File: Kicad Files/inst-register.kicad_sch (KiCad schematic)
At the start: 20 parts, among them U32 74LS245, U33 74LS173, U34 74LS173

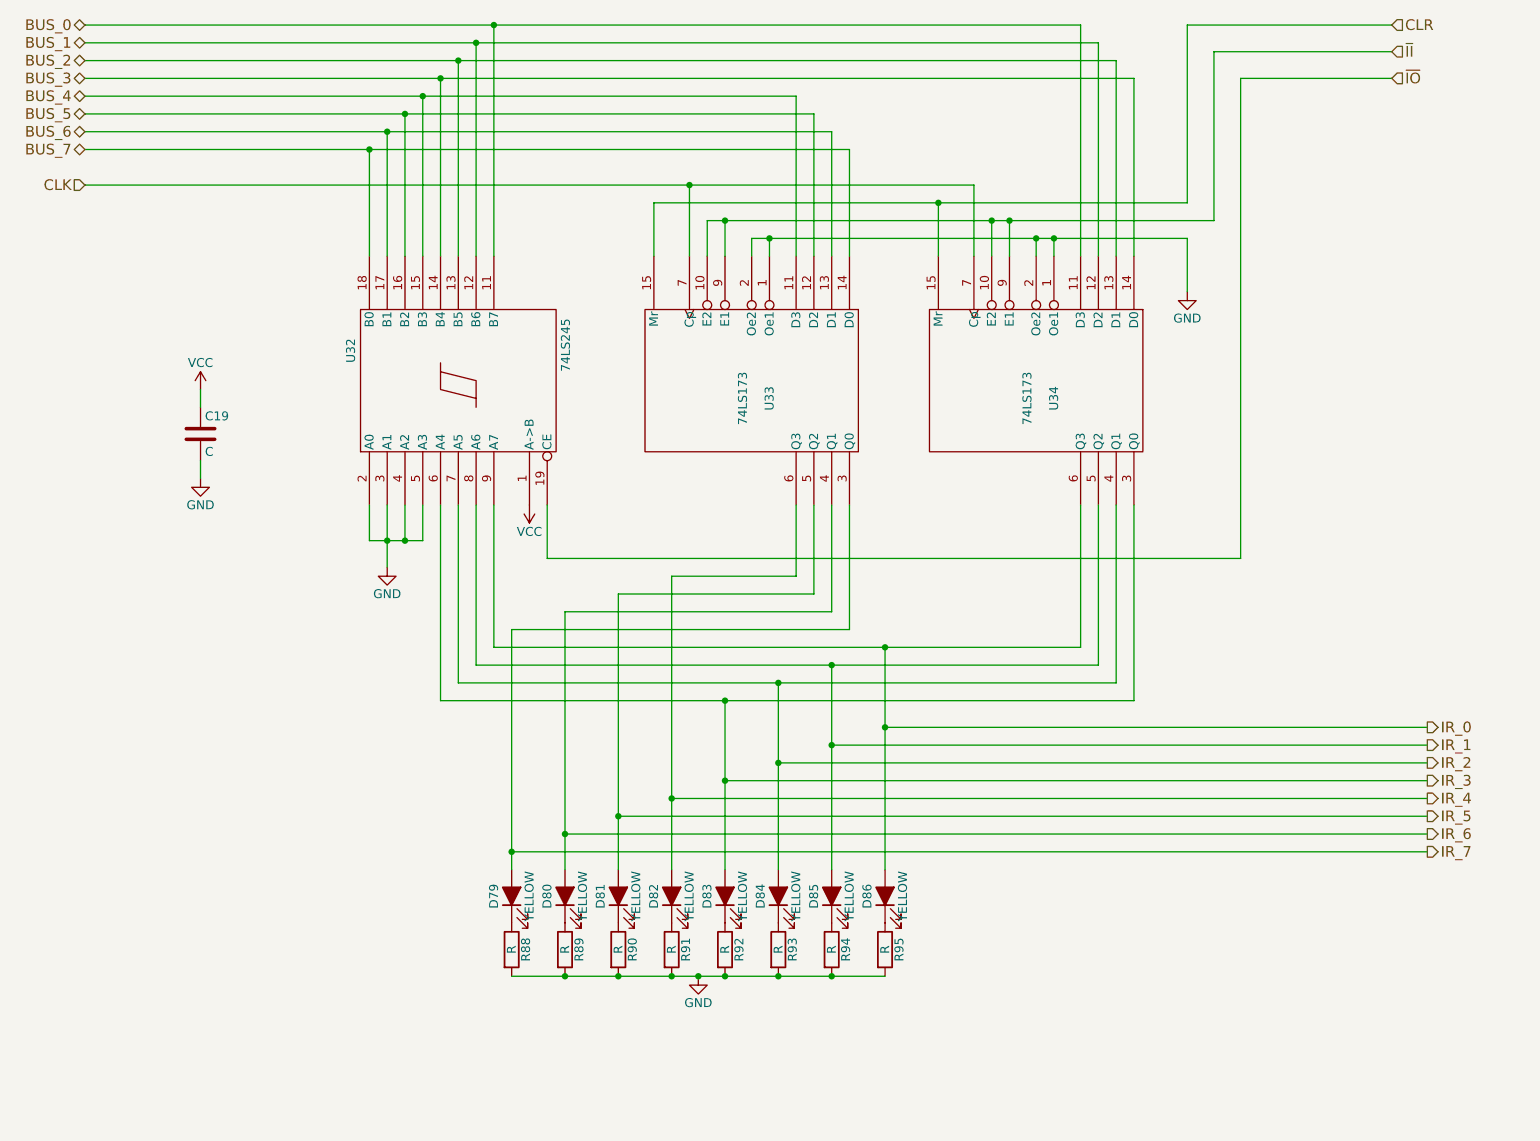
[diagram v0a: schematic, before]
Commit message: updated library
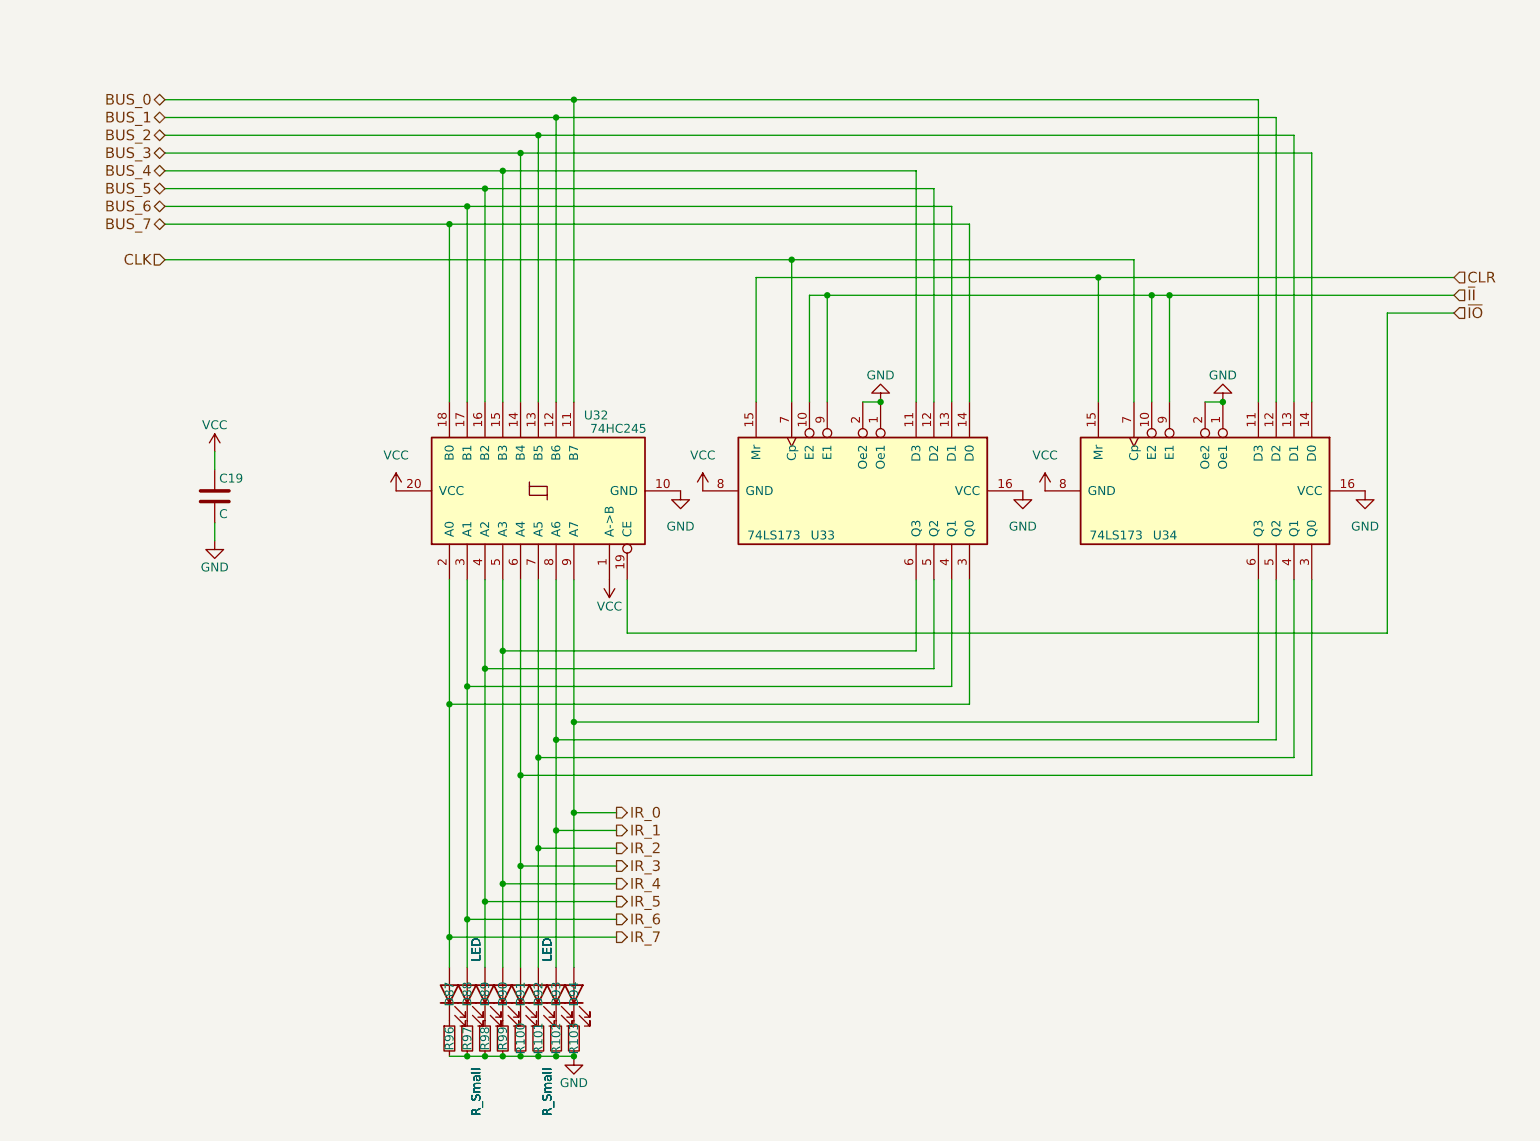
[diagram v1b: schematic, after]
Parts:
- removed D79, D80, D81, D82, D83, D84, D85, D86: YELLOW, LED_THT:LED_D5.0mm, symbol 8bit-computer-rescue:LED_ALT-Device
- removed R88, R89, R90, R91, R92, R93, R94, R95: R, Resistor_THT:R_Axial_DIN0207_L6.3mm_D2.5mm_P7.62mm_Horizontal, symbol Device:R
- removed U32: 74LS245, Package_DIP:DIP-20_W7.62mm, symbol 8bit-computer-rescue:74LS245-8bit-computer-rescue
- removed U33, U34: 74LS173, Package_DIP:DIP-16_W7.62mm, symbol 8bit-computer-rescue:74LS173-8bit-computer-rescue
- added D87, D88, D89, D90, D91, D92, D93, D94: LED, symbol Device:LED
- added R100, R101, R102, R103, R96, R97, R98, R99: R_Small, symbol Device:R_Small
- added U32: 74HC245, symbol 74xx:74HC245
- added U33, U34: 74LS173, symbol 74xx:74LS173
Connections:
- net BUS_0: now also U32.11 (B7), U34.11 (D3)
- net BUS_1: now also U32.12 (B6), U34.12 (D2)
- net BUS_2: now also U32.13 (B5), U34.13 (D1)
- net BUS_3: now also U32.14 (B4), U34.14 (D0)
- net BUS_4: now also U32.15 (B3), U33.11 (D3)
- net BUS_5: now also U32.16 (B2), U33.12 (D2)
- net BUS_6: now also U32.17 (B1), U33.13 (D1)
- net BUS_7: now also U32.18 (B0), U33.14 (D0)
- net CLK: now also U33.7 (Cp), U34.7 (Cp)
- net CLR: now also U33.15 (Mr), U34.15 (Mr)
- net GND: now also R100.2, R101.2, R102.2, R103.2, R96.2, R97.2, R98.2, R99.2, U32.10 (GND), U33.1 (Oe1), U33.16 (VCC), U33.2 (Oe2), U34.1 (Oe1), U34.16 (VCC), U34.2 (Oe2)
- net IR_0: now also D94.2 (A), U32.9 (A7), U34.6 (Q3)
- net IR_1: now also D93.2 (A), U32.8 (A6), U34.5 (Q2)
- net IR_2: now also D92.2 (A), U32.7 (A5), U34.4 (Q1)
- net IR_3: now also D91.2 (A), U32.6 (A4), U34.3 (Q0)
- net IR_4: now also D90.2 (A), U32.5 (A3), U33.6 (Q3)
- net IR_5: now also D89.2 (A), U32.4 (A2), U33.5 (Q2)
- net IR_6: now also D88.2 (A), U32.3 (A1), U33.4 (Q1)
- net IR_7: now also D87.2 (A), U32.2 (A0), U33.3 (Q0)
- net VCC: now also U32.1 (A->B), U32.20 (VCC), U33.8 (GND), U34.8 (GND)
- net ~{II}: now also U33.10 (E2), U33.9 (E1), U34.10 (E2), U34.9 (E1)
- net ~{IO}: now also U32.19 (CE)
- new net: D93.1 (K), R102.1
- new net: D87.1 (K), R96.1
- new net: D94.1 (K), R103.1
- new net: D91.1 (K), R100.1
- new net: D92.1 (K), R101.1
- new net: D88.1 (K), R97.1
- new net: D89.1 (K), R98.1
- new net: D90.1 (K), R99.1
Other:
- moved on the sheet: C19

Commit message: im sooo stupiiid
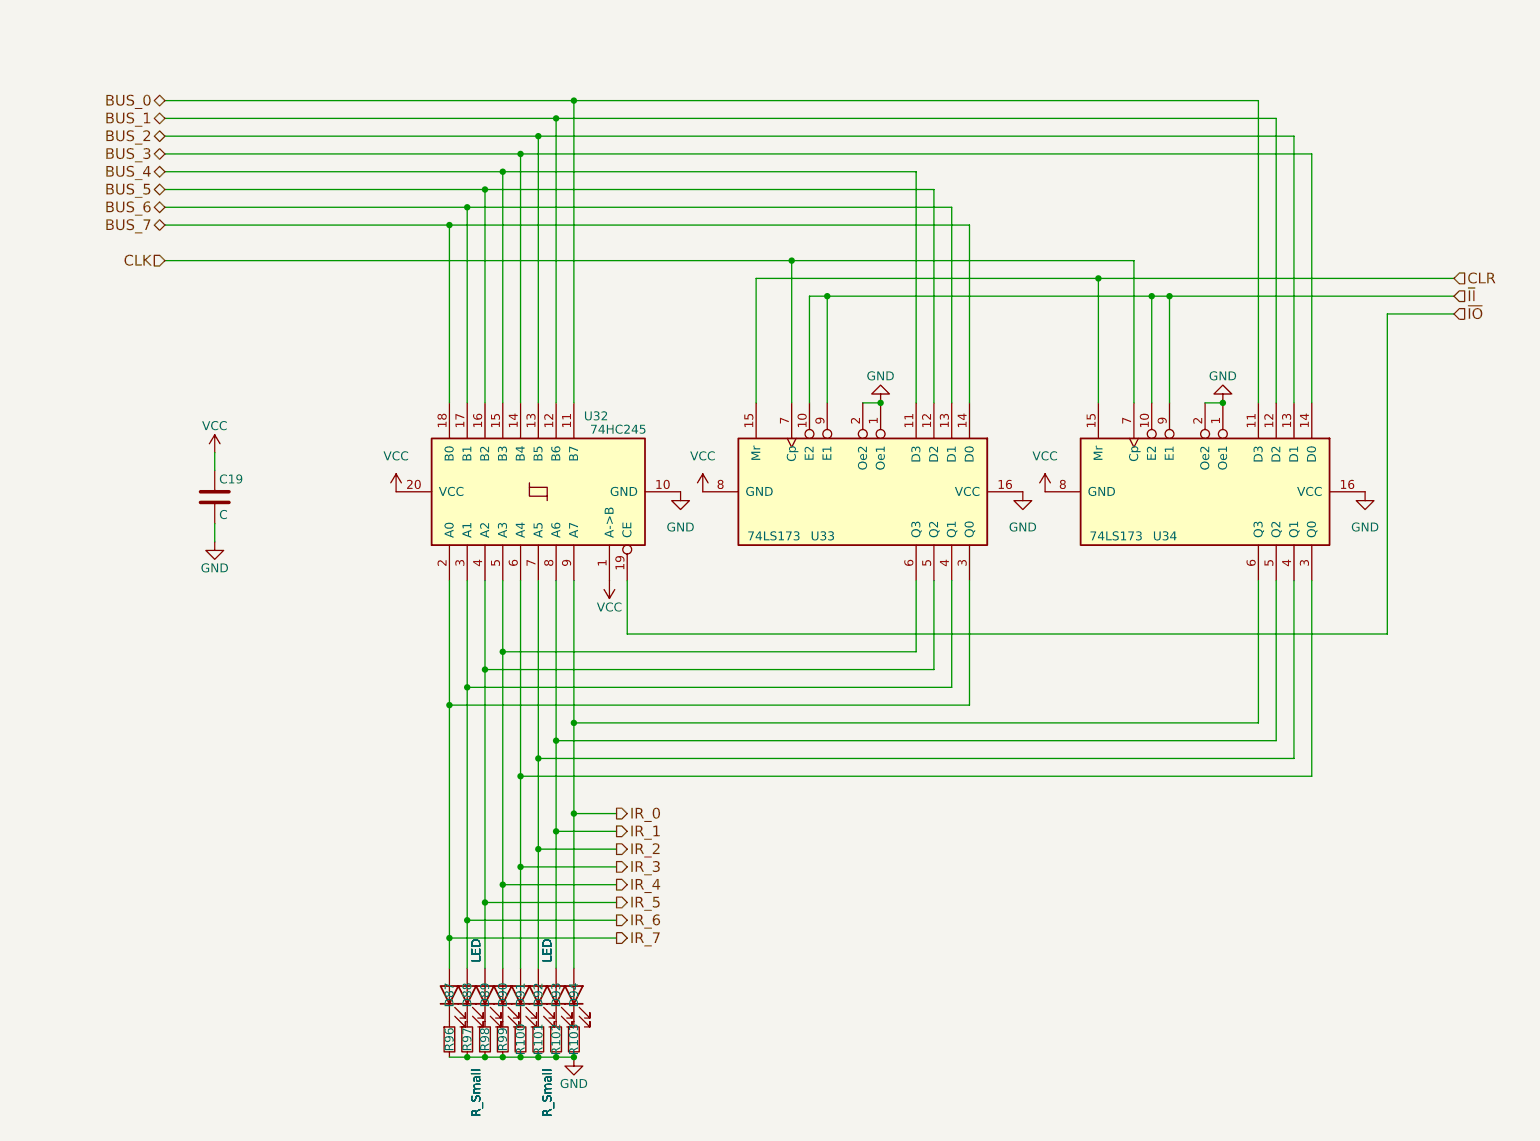
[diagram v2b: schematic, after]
